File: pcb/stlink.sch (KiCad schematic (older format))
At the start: 40 parts, among them J1 USB_A, Q1 S9013, U1 XC6206P332MR, U2 GD32F103CBT6, Y1 8MHz

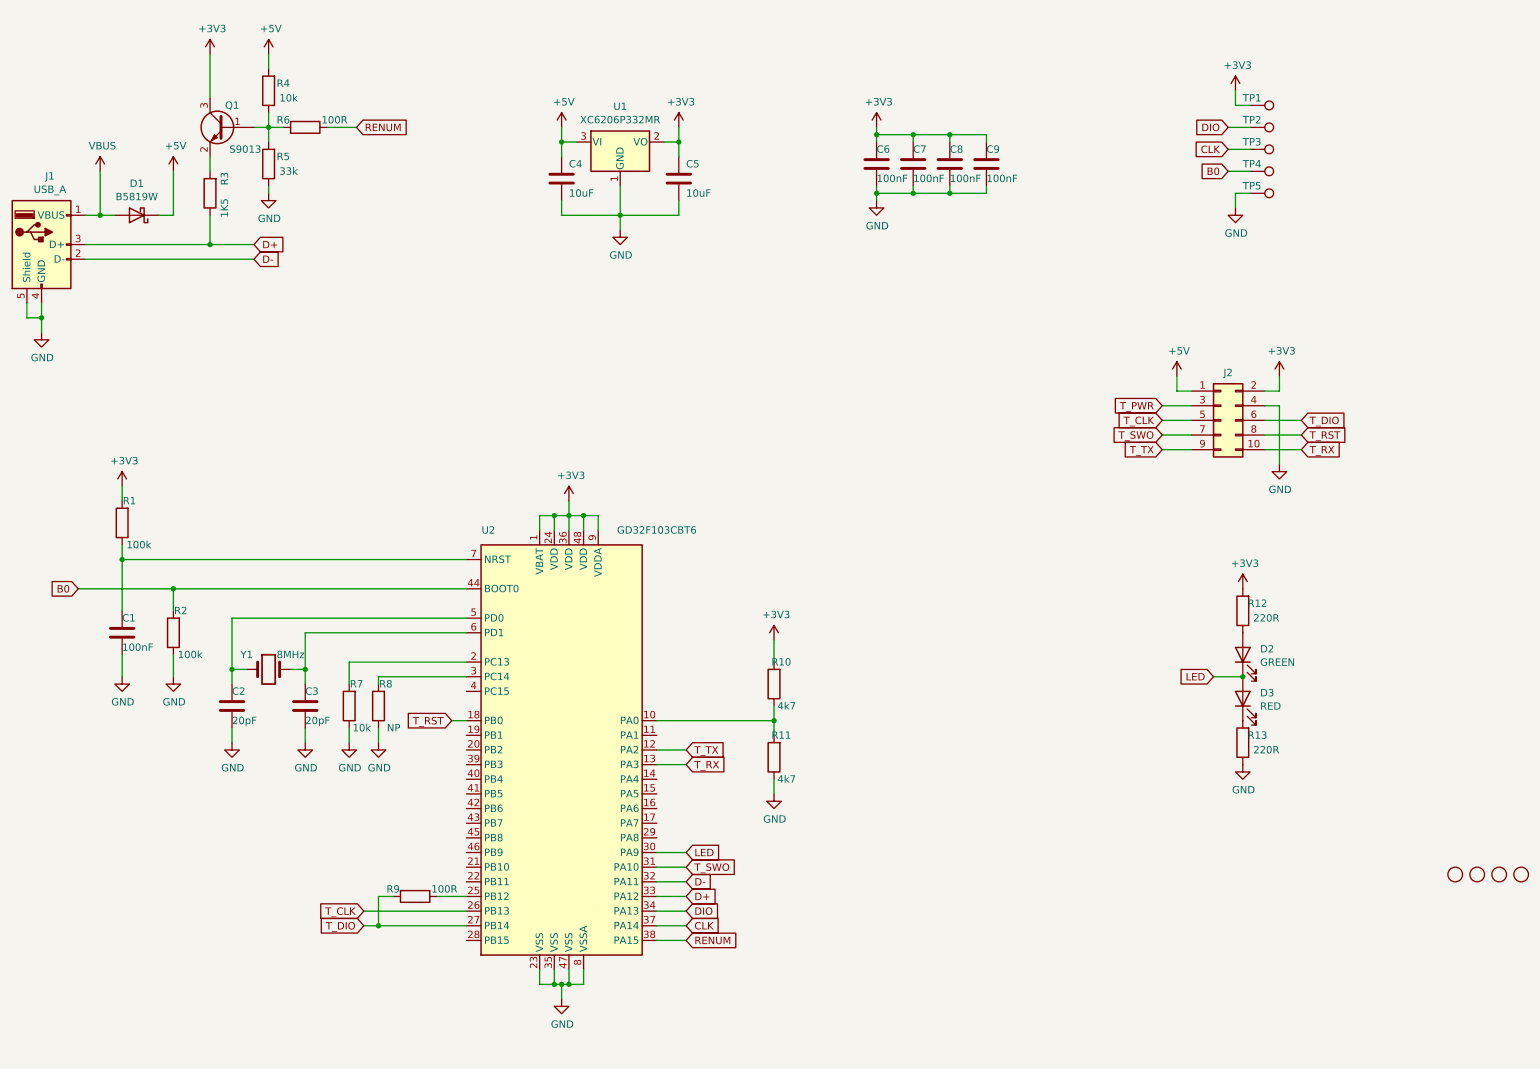
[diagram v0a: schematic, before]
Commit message: Hmmm
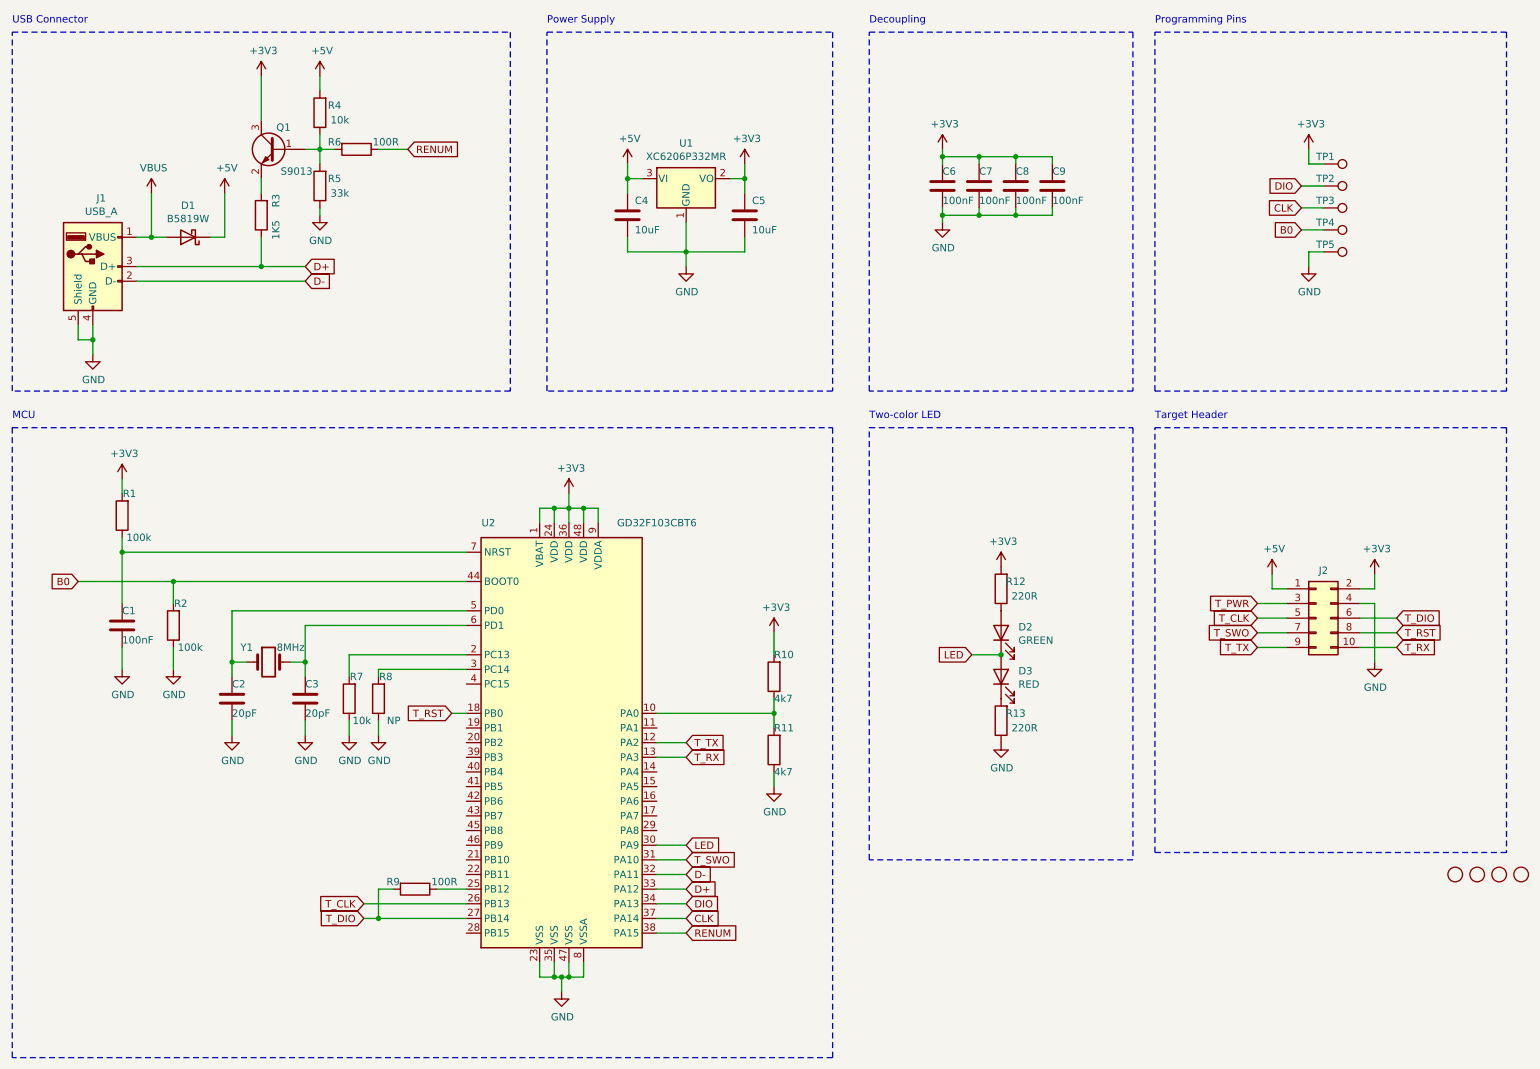
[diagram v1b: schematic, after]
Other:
- note added: "Decoupling"
- note added: "MCU"
- note added: "Power Supply"
- note added: "Programming Pins"
- note added: "Target Header"
- note added: "Two-color LED"
- note added: "USB Connector"
- moved on the sheet: C1, C2, C3, C4, C5, C6, C7, C8, C9, D1, D2, D3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
